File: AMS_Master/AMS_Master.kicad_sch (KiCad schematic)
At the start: 13 parts, among them IC1 LTM2884CY#PBF, IC2 LTC4411ES5#TRMPBF, IC3 ISO1042DWVR, J1 Conn_01x04_Socket, J2 Conn_01x04_Socket, J3 USB_B, U1 LD1117S50TR_SOT223, U2 ADuM1250, U3 MCP2515-xSO, Y1 Crystal

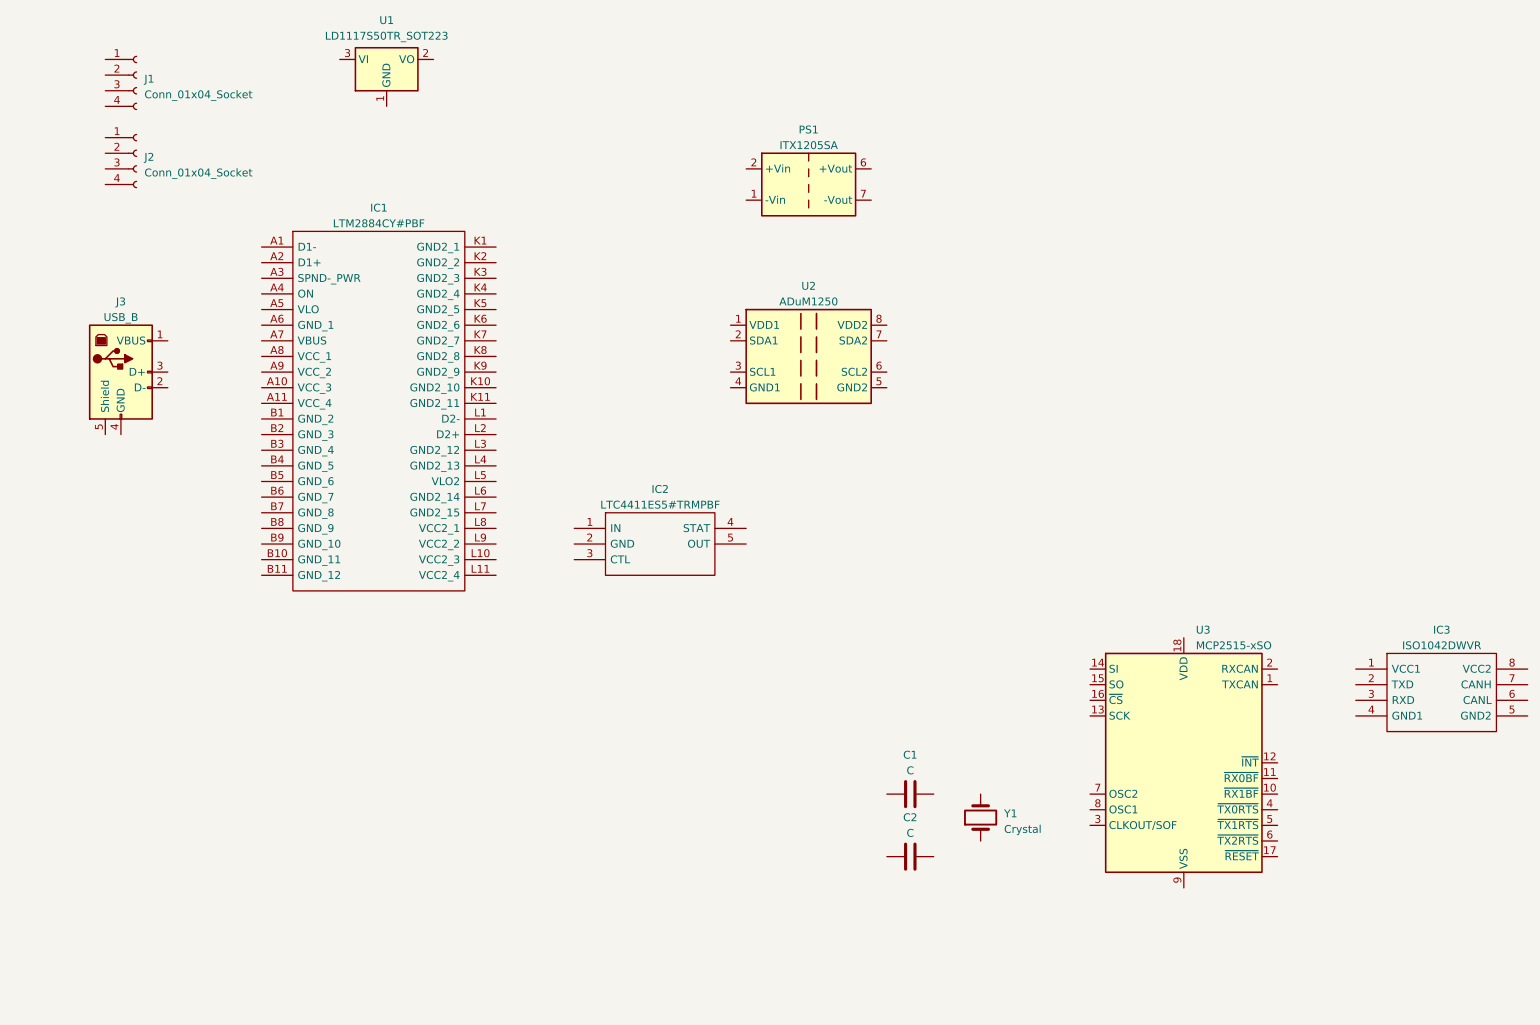
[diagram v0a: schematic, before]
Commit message: AMS_Master更新
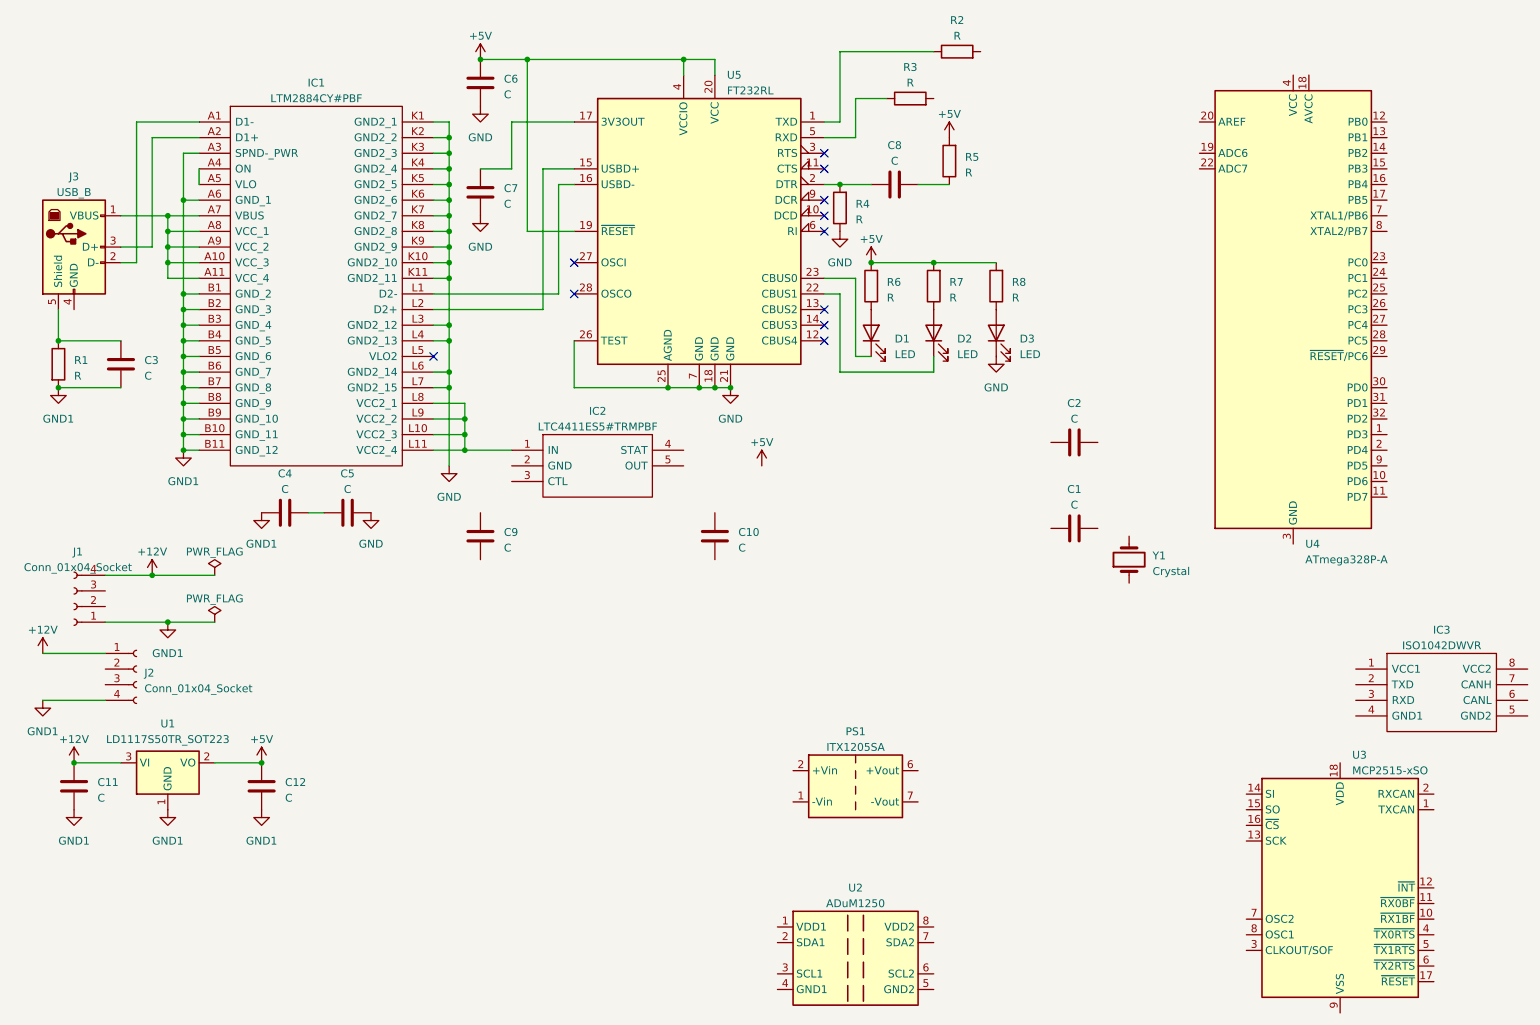
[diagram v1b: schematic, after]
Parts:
- added C10, C11, C12, C3, C4, C5, C6, C7, C8, C9: C, symbol Device:C
- added D1, D2, D3: LED, symbol Device:LED
- added R1, R2, R3, R4, R5, R6, R7, R8: R, symbol Device:R
- added U4: ATmega328P-A, Package_QFP:TQFP-32_7x7mm_P0.8mm, symbol MCU_Microchip_ATmega:ATmega328P-A
- added U5: FT232RL, Package_SO:SSOP-28_5.3x10.2mm_P0.65mm, symbol Interface_USB:FT232RL
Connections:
- net GND1: now reaches U1.1 (GND)
- net GND1: now also IC1.A3 (SPND-_PWR), IC1.A6 (GND_1), IC1.B1 (GND_2), IC1.B10 (GND_11), IC1.B11 (GND_12), IC1.B2 (GND_3), IC1.B3 (GND_4), IC1.B4 (GND_5), IC1.B5 (GND_6), IC1.B6 (GND_7), IC1.B7 (GND_8), IC1.B8 (GND_9), IC1.B9 (GND_10), J1.1 (Pin_1), J2.4 (Pin_4), C11.2, C12.2, C3.2, C4.1, R1.2
- net +5V: now reaches U1.2 (VO)
- net +5V: now also C12.1, C6.1, R5.2, R6.2, R7.2, R8.2, U5.19 (~{RESET}), U5.20 (VCC), U5.4 (VCCIO)
- net +12V: now reaches U1.3 (VI)
- net +12V: now also J1.4 (Pin_4), J2.1 (Pin_1), C11.1
- net at IC1.A1 (D1-): now also J3.2 (D-)
- net at IC1.A10 (VCC_3): now also IC1.A11 (VCC_4), IC1.A7 (VBUS), IC1.A8 (VCC_1), IC1.A9 (VCC_2), J3.1 (VBUS)
- net at IC1.A2 (D1+): now also J3.3 (D+)
- net at IC1.A4 (ON): now also IC1.A5 (VLO)
- net GND: now reaches IC1.K1 (GND2_1)
- net GND: now also IC1.K10 (GND2_10), IC1.K11 (GND2_11), IC1.K2 (GND2_2), IC1.K3 (GND2_3), IC1.K4 (GND2_4), IC1.K5 (GND2_5), IC1.K6 (GND2_6), IC1.K7 (GND2_7), IC1.K8 (GND2_8), IC1.K9 (GND2_9), IC1.L3 (GND2_12), IC1.L4 (GND2_13), IC1.L6 (GND2_14), IC1.L7 (GND2_15), C5.2, C6.2, C7.2, D3.1 (K), R4.1, U5.18 (GND), U5.21 (GND), U5.25 (AGND), U5.26 (TEST), U5.7 (GND)
- net at IC1.L1 (D2-): now also U5.16 (USBD-)
- net at IC1.L10 (VCC2_3): now also IC1.L11 (VCC2_4), IC1.L8 (VCC2_1), IC1.L9 (VCC2_2), IC2.1 (IN)
- net at IC1.L2 (D2+): now also U5.15 (USBD+)
- net at J3.5 (Shield): now also C3.1, R1.1
- new net: C4.2, C5.1
- new net: C8.2, R5.1
- new net: D3.2 (A), R8.1
- new net: C8.1, R4.2, U5.2 (DTR)
- new net: R3.1, U5.5 (RXD)
- new net: C7.1, U5.17 (3V3OUT)
- new net: D1.1 (K), U5.23 (CBUS0)
- new net: D1.2 (A), R6.1
- new net: D2.2 (A), R7.1
- new net: U4.21 (GND), U4.3 (GND), U4.5 (GND)
- new net: U4.4 (VCC), U4.6 (VCC)
- new net: R2.1, U5.1 (TXD)
- new net: D2.1 (K), U5.22 (CBUS1)
- no-connect marks 0 -> 11
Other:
- moved on the sheet: C1, C2, IC1, IC2, J1, J2, J3, PS1, U1, U2, U3, Y1
